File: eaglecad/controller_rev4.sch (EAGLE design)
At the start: 96 parts, among them J1 1.27MM-SWD-CONNECTOR, U101 TCAN330, U200 TPS63070, U300 STSPIN230, U301 TSV991ILT, U302 AS5047P, U400 STSPIN250, U401 TSV991ILT, X101 16MHZ-2.5x2mm

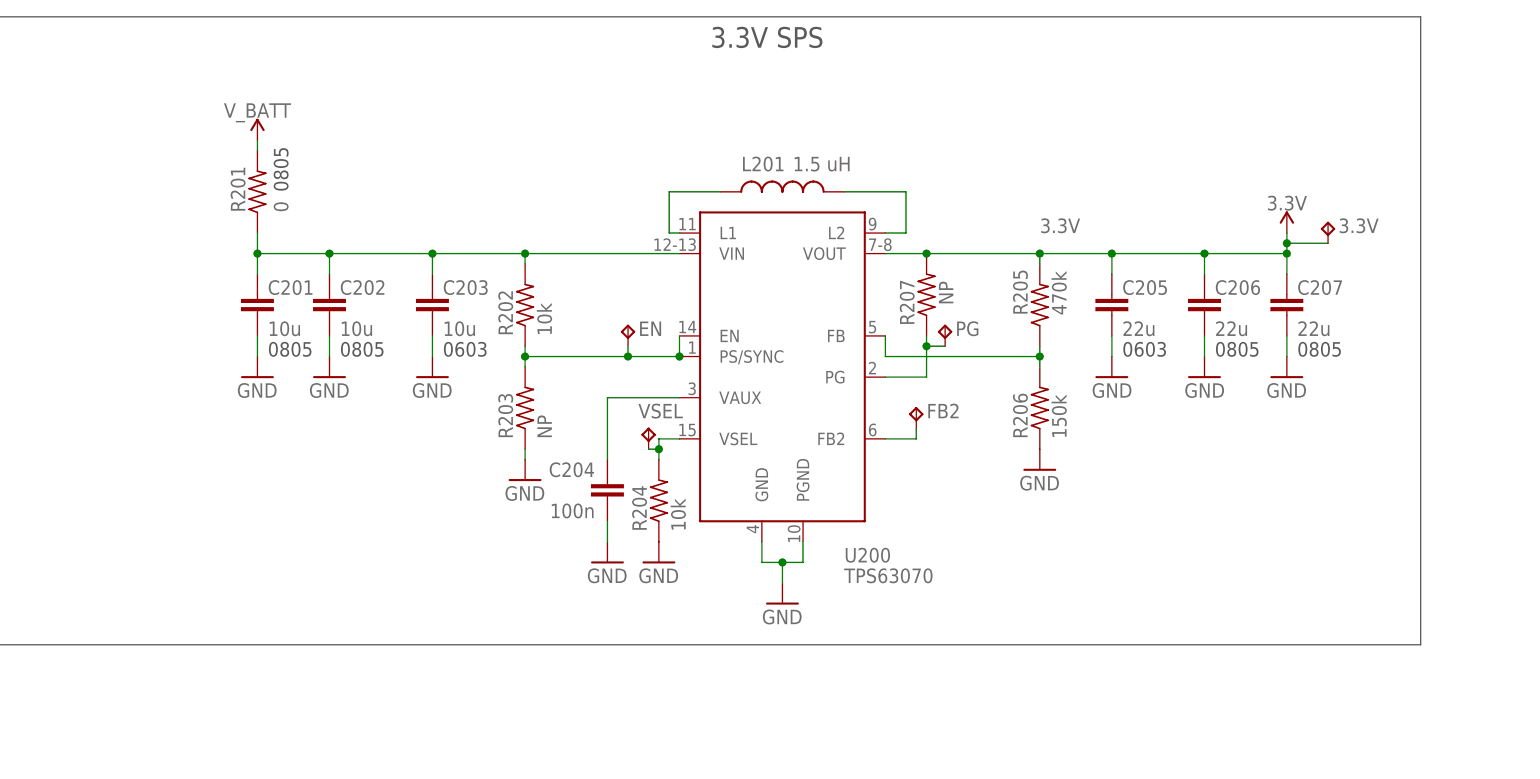
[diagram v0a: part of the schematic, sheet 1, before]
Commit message: F4 update
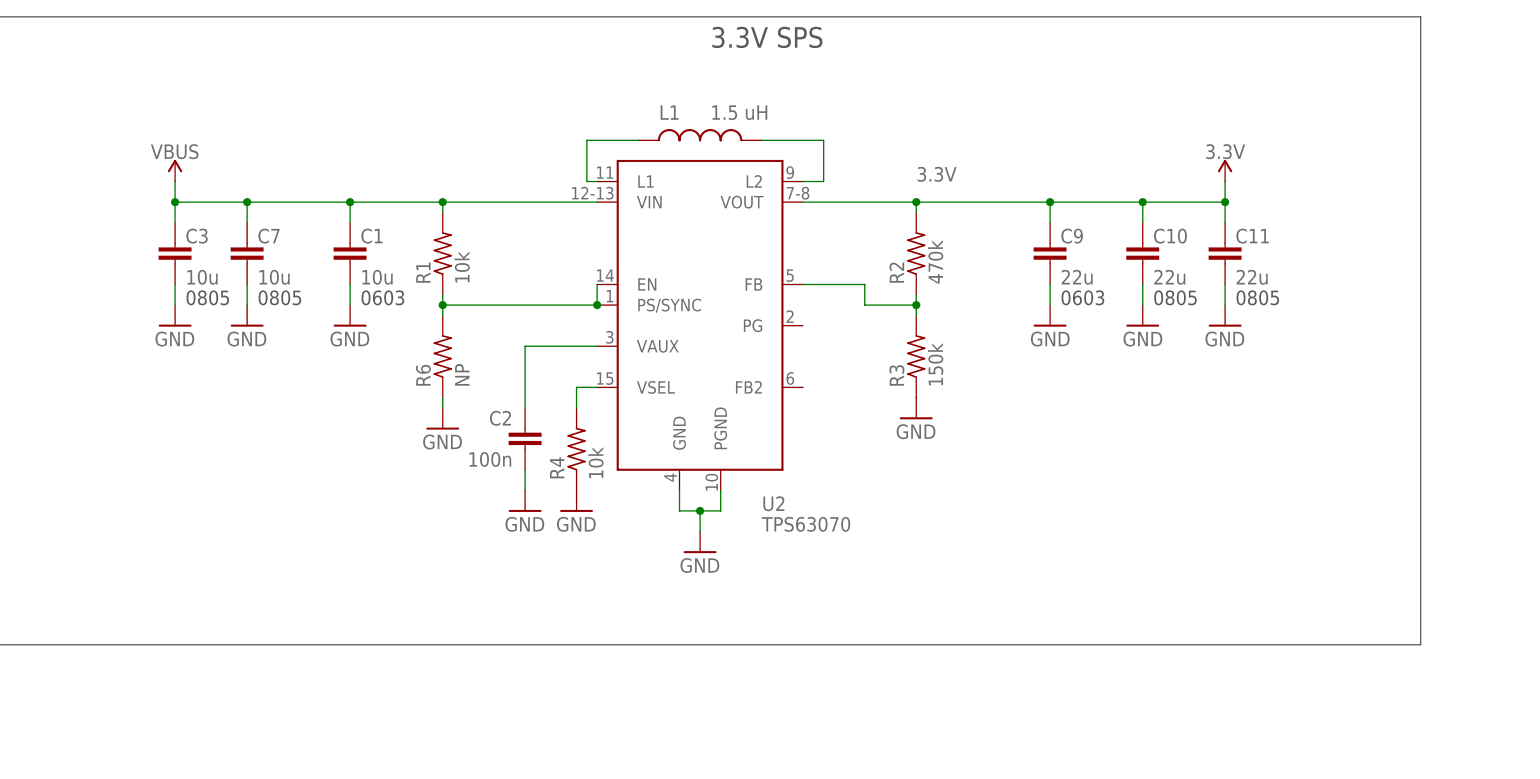
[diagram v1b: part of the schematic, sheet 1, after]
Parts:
- removed 3.3V, EN, FB2, PG, VSEL: TPTP15SQ, testpad:TPTP15SQ
- removed C201, C202: 10u, oresat-rcl:C-EU0805-B-NOSILK
- removed C203: 10u, oresat-rcl:C-EU0603-B-NOSILK
- removed C204: 100n, rcl_custom:C-EU0402-B-NOSILK
- removed C205: 22u, oresat-rcl:C-EU0603-B-NOSILK
- removed C206, C207: 22u, oresat-rcl:C-EU0805-B-NOSILK
- removed L201: 1.5 uH, L-Coilcraft-XFL4020:L-COILCRAFT-XFL4020
- removed R201: 0, rcl_custom:R-US_0805-B-NOSILK
- removed R202, R204: 10k, rcl_custom:R-US_0402-B-NOSILK
- removed R203, R207: NP, rcl_custom:R-US_0402-B-NOSILK
- removed R205: 470k, rcl_custom:R-US_0402-B-NOSILK
- removed R206: 150k, rcl_custom:R-US_0402-B-NOSILK
- removed U200: TPS63070, ic-pwr-tps63070x:TPS63070X
- added C1: 10u, oresat-rcl:C-EU0603-B-NOSILK
- added C10, C11: 22u, oresat-rcl:C-EU0805-B-NOSILK
- added C2: 100n, rcl_custom:C-EU0402-B-NOSILK
- added C3, C7: 10u, oresat-rcl:C-EU0805-B-NOSILK
- added C9: 22u, oresat-rcl:C-EU0603-B-NOSILK
- added L1: 1.5 uH, L-Coilcraft-XFL4020:L-COILCRAFT-XFL4020
- added R1, R4: 10k, rcl_custom:R-US_0402-B-NOSILK
- added R2: 470k, rcl_custom:R-US_0402-B-NOSILK
- added R3: 150k, rcl_custom:R-US_0402-B-NOSILK
- added R6: NP, rcl_custom:R-US_0402-B-NOSILK
- added U2: TPS63070, ic-pwr-tps63070x:TPS63070X
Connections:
- removed net TPS-EN: EN.TP, R202.1, R203.2, U200.EN, U200.PS/SYNC
- removed net TPS-FB: R205.1, R206.2, U200.FB
- removed net TPS-L1: L201.1, U200.L1
- removed net TPS-L2: L201.2, U200.L2
- removed net TPS-PG: PG.TP, R207.1, U200.PG
- removed net TPS-VAUX: C204.1, U200.VAUX
- removed net TPS-VIN: C201.1, C202.1, C203.1, R201.1, R202.2, U200.VIN
- removed net TSP-FB2: FB2.TP, U200.FB2
- removed net TSP-VSEL: R204.2, U200.VSEL, VSEL.TP
- new net TPS-EN2: R1.1, R6.2, U2.EN, U2.PS/SYNC
- new net TPS-FB2: R2.1, R3.2, U2.FB
- new net TPS-L5: L1.1, U2.L1
- new net TPS-L6: L1.2, U2.L2
- new net TPS-VAUX2: C2.1, U2.VAUX
- new net TPS-VSEL2: R4.2, U2.VSEL
- new net VBUS: C1.1, C3.1, C7.1, R1.2, U2.VIN
- net 3.3V: now also C10.1, C11.1, C9.1, R2.2, U2.VOUT; no longer 3.3V.TP, C205.1, C206.1, C207.1, R205.2, R207.2, U200.VOUT
- net GND: now also C1.2, C10.2, C11.2, C2.2, C3.2, C7.2, C9.2, R3.1, R4.1, R6.1, U2.GND, U2.PGND; no longer C201.2, C202.2, C203.2, C204.2, C205.2, C206.2, C207.2, R203.1, R204.1, R206.1, U200.GND, U200.PGND
- net V_BATT: no longer R201.2

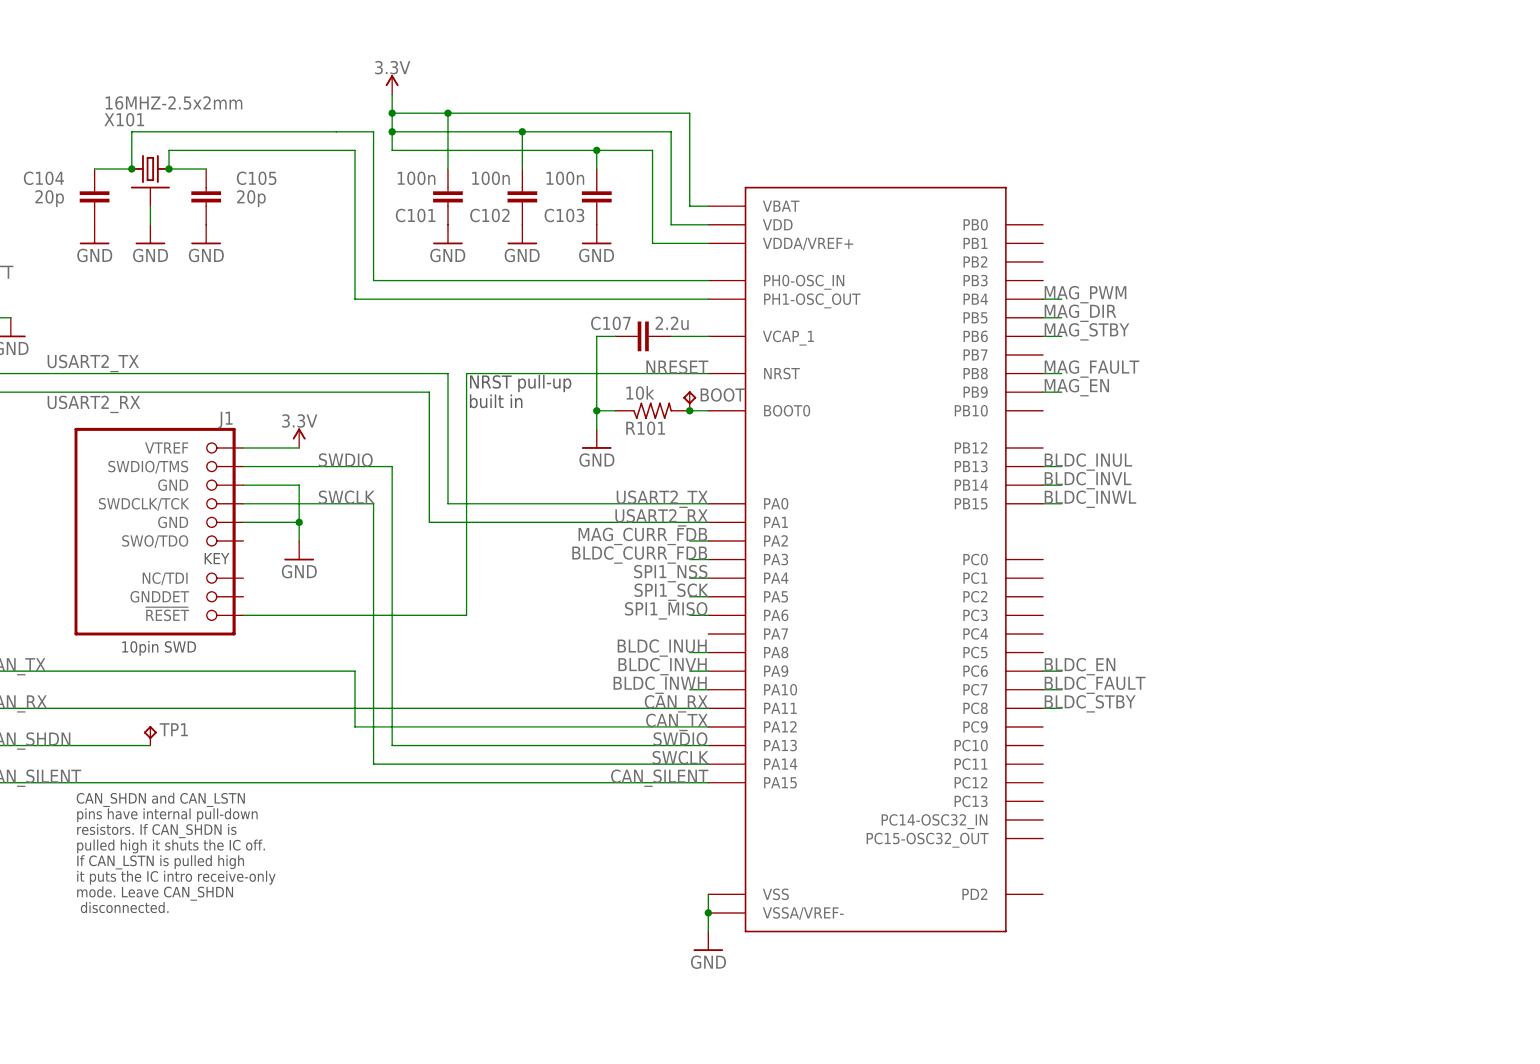
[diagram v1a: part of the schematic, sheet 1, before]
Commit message: L4 updates
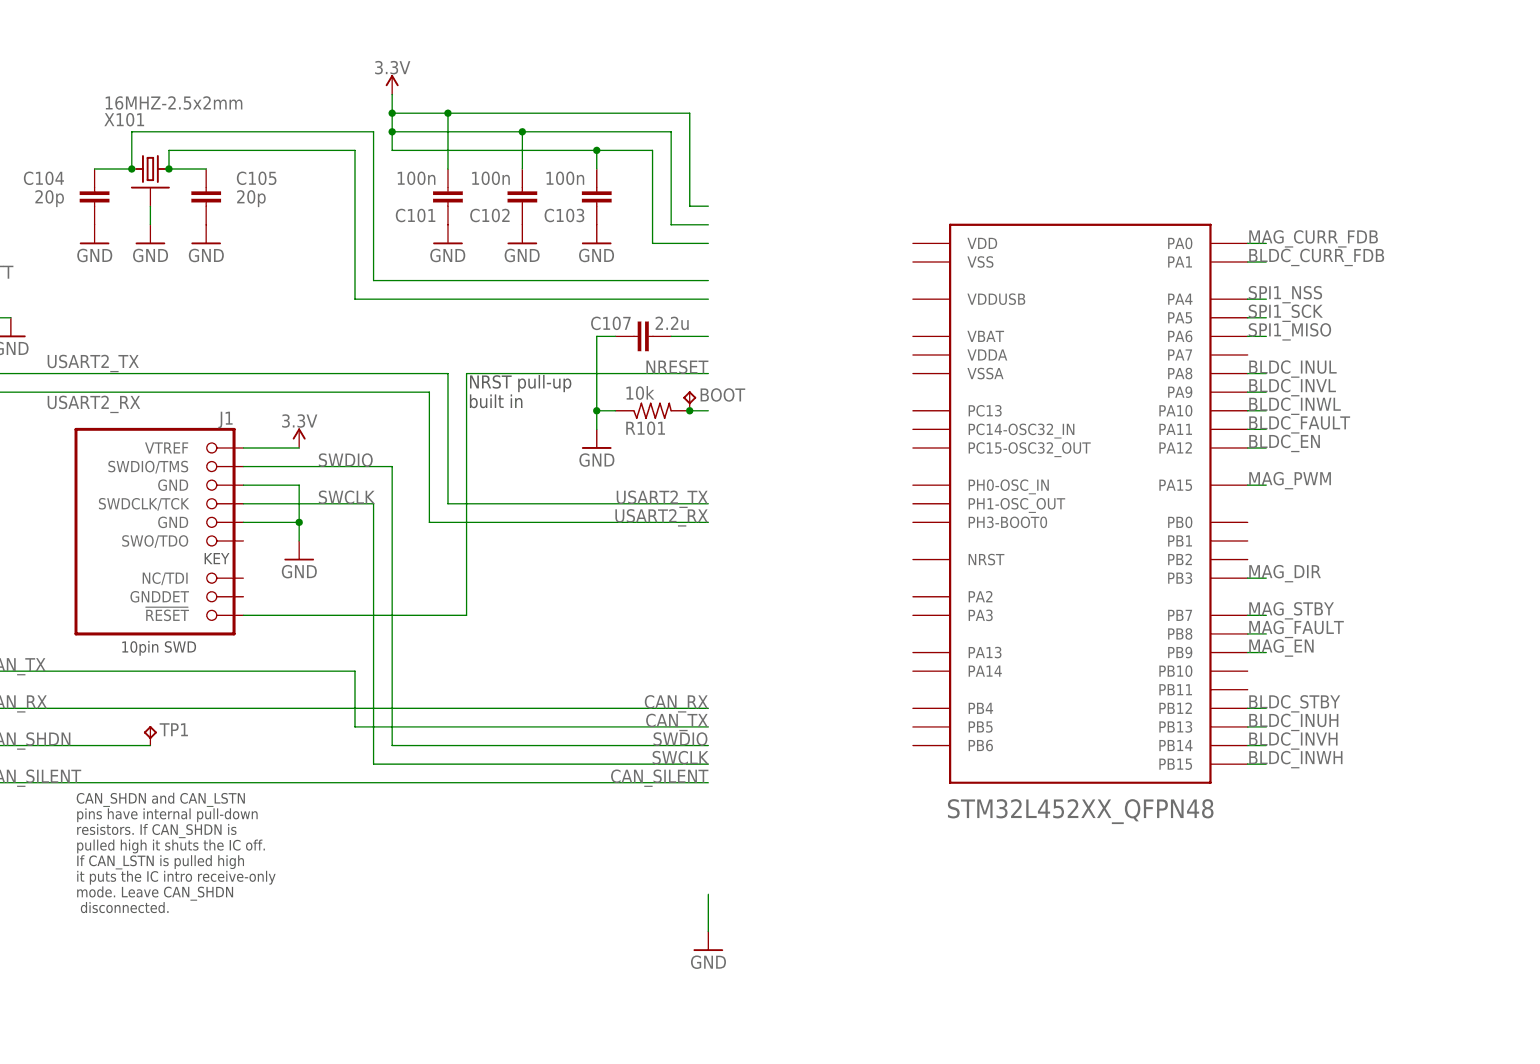
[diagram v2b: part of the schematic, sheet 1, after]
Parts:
- U$1: value STM32F446X -> STM32L452XX_QFPN48; device oresat-misc:STM32F446X -> oresat-ACS_driver_board:STM32L452XX_QFPN48
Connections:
- net 3.3V: no longer U$1.VBAT, U$1.VDD, U$1.VDDA/VREF+
- net BLDC_CURR_FDB: now also U$1.PA1; no longer U$1.PA3
- net BLDC_EN: now also U$1.PA12; no longer U$1.PC6
- net BLDC_FAULT: now also U$1.PA11; no longer U$1.PC7
- net BLDC_INUH: now also U$1.PB13; no longer U$1.PA8
- net BLDC_INUL: now also U$1.PA8; no longer U$1.PB13
- net BLDC_INVH: now also U$1.PB14; no longer U$1.PA9
- net BLDC_INVL: now also U$1.PA9; no longer U$1.PB14
- net BLDC_INWH: now also U$1.PB15; no longer U$1.PA10
- net BLDC_INWL: now also U$1.PA10; no longer U$1.PB15
- net BLDC_STBY: now also U$1.PB12; no longer U$1.PC8
- net BOOT: no longer U$1.BOOT0
- net CAN_RX: no longer U$1.PA11
- net CAN_SILENT: no longer U$1.PA15
- net CAN_TX: no longer U$1.PA12
- net GND: no longer U$1.VSS, U$1.VSSA/VREF-
- net MAG_CURR_FDB: now also U$1.PA0; no longer U$1.PA2
- net MAG_DIR: now also U$1.PB3; no longer U$1.PB5
- net MAG_PWM: now also U$1.PA15; no longer U$1.PB4
- net MAG_STBY: now also U$1.PB7; no longer U$1.PB6
- net N$1: no longer U$1.PH0-OSC_IN
- net N$4: no longer U$1.PH1-OSC_OUT
- net N$6: no longer U$1.VCAP_1
- net NRESET: no longer U$1.NRST
- net SWCLK: no longer U$1.PA14
- net SWDIO: no longer U$1.PA13
- net USART2_RX: no longer U$1.PA1
- net USART2_TX: no longer U$1.PA0
